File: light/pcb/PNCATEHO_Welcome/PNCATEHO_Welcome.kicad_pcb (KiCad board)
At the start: 2 copper layers, 85.6 x 54 mm, 61 parts, among them J1 USB_C_Receptacle_USB2.0, SW11 Boot, SW12 Reset, U1 RP2040, U2 RT9013-33GB, U3 W25Q32JVSSIQ, U4 USBLC6-2SC6, Y1 12MHz

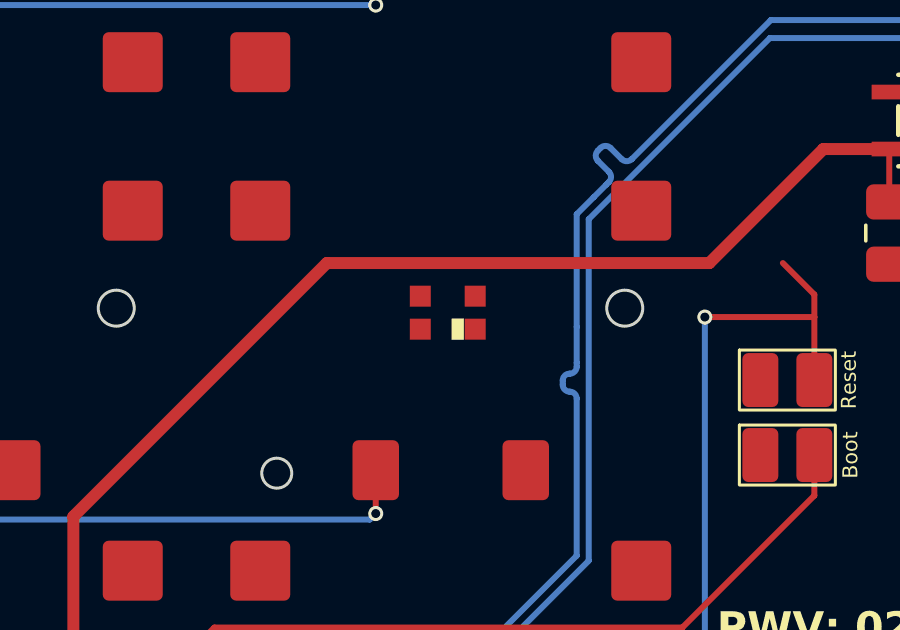
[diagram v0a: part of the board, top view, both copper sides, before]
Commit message: fix sh
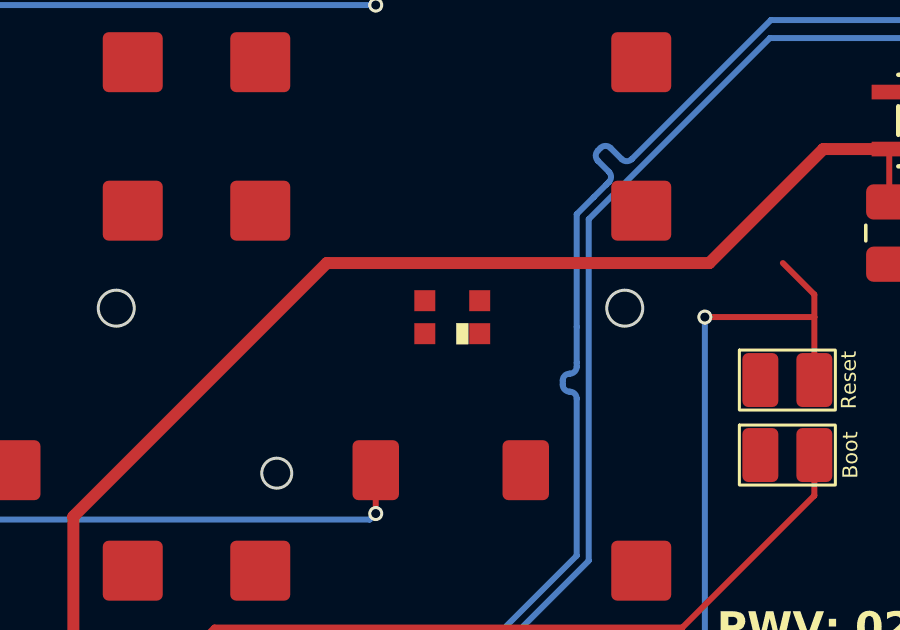
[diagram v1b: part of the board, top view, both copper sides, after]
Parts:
- D10, D11, D12, D3, D4, D5, D6, D7, D8, D9: value LED_WS2812-2020 -> ~
- moved D3 50.9 mm to (156.7, 82.8)
- moved D6 50.9 mm to (105.9, 82.8)
- moved D4 16.9 mm to (139.8, 82.8)
- moved D5 16.9 mm to (122.8, 82.8)
- moved D10 0.21 mm to (156.7, 99.8)
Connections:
- D11 pad 1: Net-(D10-DI) -> Net-(D11-DO)
- D11 pad 3: Net-(D11-DI) -> Net-(D10-DO)
- D12 pad 1: Net-(D11-DI) -> unconnected-(D12-DO-Pad1)
- D12 pad 3: unconnected-(D12-DI-Pad3) -> Net-(D11-DO)
- D3 pad 3: Net-(D3-DI) -> LED
- D4 pad 1: Net-(D3-DI) -> Net-(D4-DO)
- D4 pad 3: Net-(D4-DI) -> Net-(D3-DO)
- D5 pad 1: Net-(D4-DI) -> Net-(D5-DO)
- D5 pad 3: Net-(D5-DI) -> Net-(D4-DO)
- D6 pad 1: LED -> Net-(D6-DO)
- D6 pad 3: Net-(D3-DO) -> Net-(D5-DO)
- D7 pad 1: Net-(D5-DI) -> Net-(D7-DO)
- D7 pad 3: Net-(D7-DI) -> Net-(D6-DO)
- D8 pad 1: Net-(D7-DI) -> Net-(D8-DO)
- D8 pad 3: Net-(D8-DI) -> Net-(D7-DO)
- D9 pad 1: Net-(D8-DI) -> Net-(D10-DI)
- D9 pad 3: Net-(D10-DO) -> Net-(D8-DO)
